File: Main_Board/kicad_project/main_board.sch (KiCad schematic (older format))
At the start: 0 parts

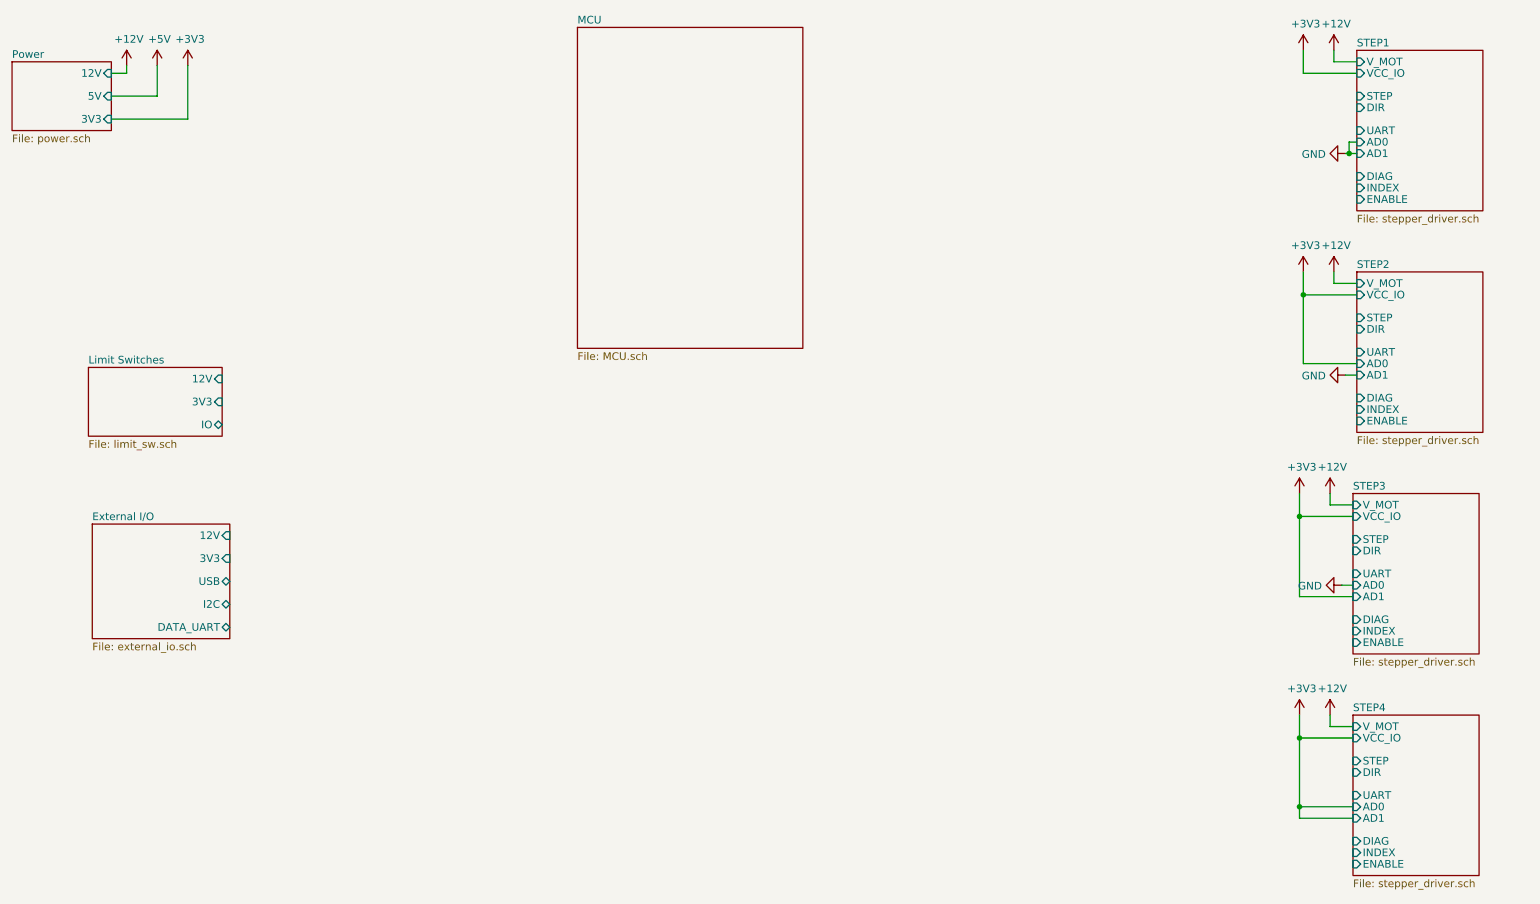
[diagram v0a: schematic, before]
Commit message: progress?
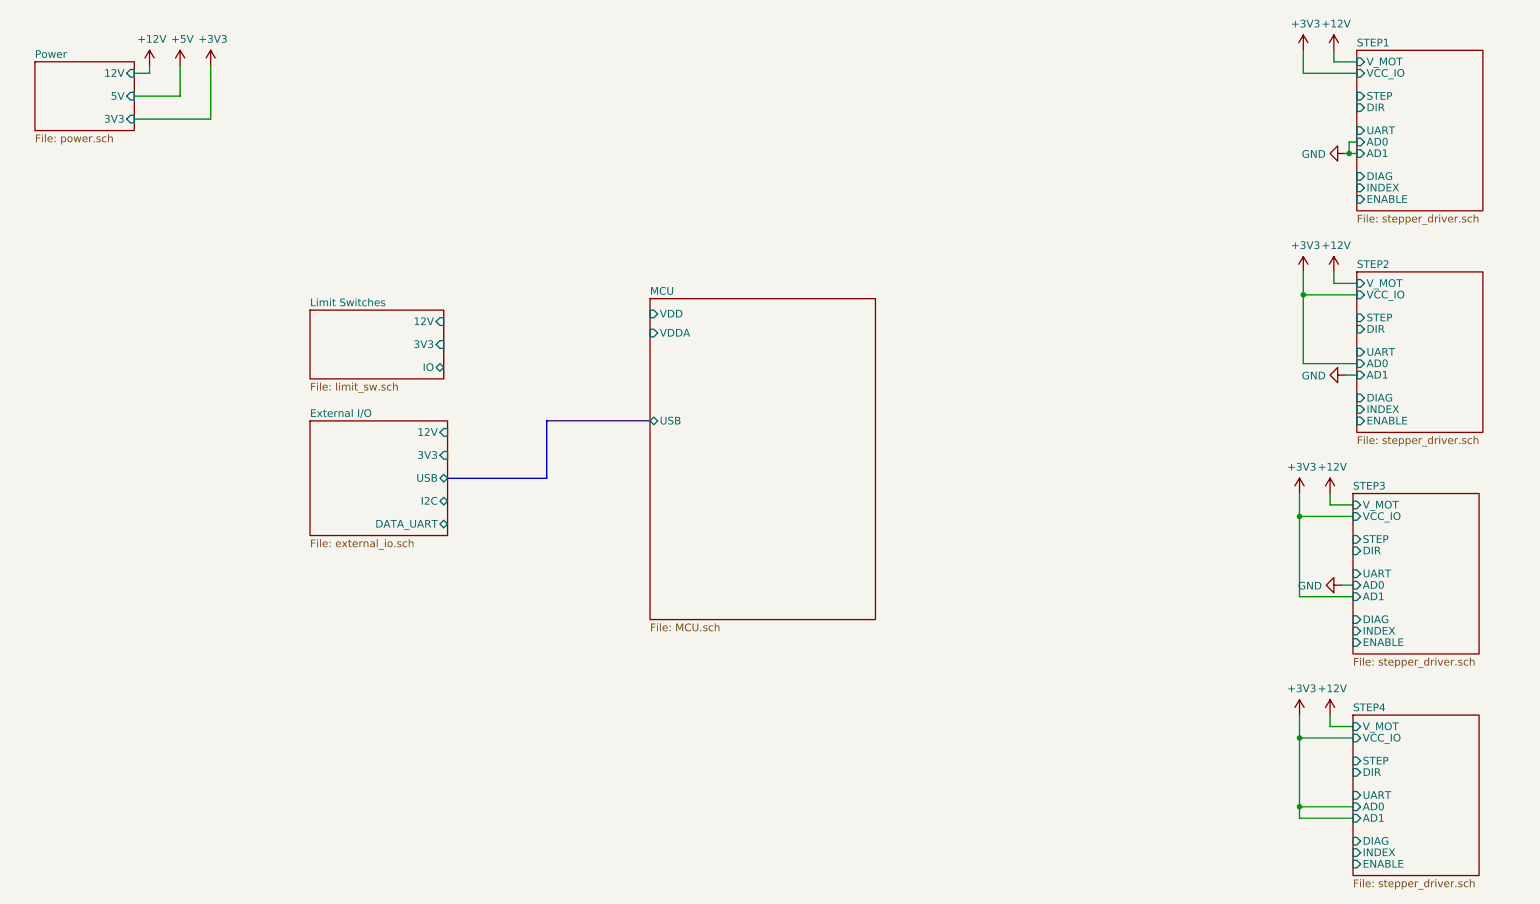
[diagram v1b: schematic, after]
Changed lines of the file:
@@
 	9500 1000 9500 850
 $Comp
-L power:+3V3 #PWR?
+L power:+3V3 #PWR06
 U 1 1 5F4AAFEB
 P 9500 850
-F 0 "#PWR?" H 9500 700 50  0001 C CNN
+F 0 "#PWR06" H 9500 700 50  0001 C CNN
 F 1 "+3V3" H 9515 1023 50  0000 C CNN
 F 2 "" H 9500 850 50  0001 C CNN
@@
 	9500 2450 9500 2300
 $Comp
-L power:+3V3 #PWR?
+L power:+3V3 #PWR07
 U 1 1 5F4AC7A4
 P 9500 2300
-F 0 "#PWR?" H 9500 2150 50  0001 C CNN
+F 0 "#PWR07" H 9500 2150 50  0001 C CNN
 F 1 "+3V3" H 9515 2473 50  0000 C CNN
 F 2 "" H 9500 2300 50  0001 C CNN
@@
 	9475 3900 9475 3750
 $Comp
-L power:+3V3 #PWR?
+L power:+3V3 #PWR04
 U 1 1 5F4AD226
 P 9475 3750
-F 0 "#PWR?" H 9475 3600 50  0001 C CNN
+F 0 "#PWR04" H 9475 3600 50  0001 C CNN
 F 1 "+3V3" H 9490 3923 50  0000 C CNN
 F 2 "" H 9475 3750 50  0001 C CNN
@@
 	9475 5350 9475 5200
 $Comp
-L power:+3V3 #PWR?
+L power:+3V3 #PWR05
 U 1 1 5F4ADFB4
 P 9475 5200
-F 0 "#PWR?" H 9475 5050 50  0001 C CNN
+F 0 "#PWR05" H 9475 5050 50  0001 C CNN
 F 1 "+3V3" H 9490 5373 50  0000 C CNN
 F 2 "" H 9475 5200 50  0001 C CNN
@@
 $EndComp
 $Sheet
-S 1050 925  650  450
+S 1200 925  650  450
 U 5F4D5F3E
 F0 "Power" 50
 F1 "power.sch" 50
-F2 "3V3" I R 1700 1300 50
-F3 "12V" I R 1700 1000 50
-F4 "5V" I R 1700 1150 50
-$EndSheet
-$Comp
-L power:+12V #PWR?
+F2 "3V3" I R 1850 1300 50
+F3 "12V" I R 1850 1000 50
+F4 "5V" I R 1850 1150 50
+$EndSheet
+$Comp
+L power:+12V #PWR09
 U 1 1 5F5780D9
 P 9675 5200
-F 0 "#PWR?" H 9675 5050 50  0001 C CNN
+F 0 "#PWR09" H 9675 5050 50  0001 C CNN
 F 1 "+12V" H 9690 5373 50  0000 C CNN
 F 2 "" H 9675 5200 50  0001 C CNN
@@
 $EndComp
 $Comp
-L power:+12V #PWR?
+L power:+12V #PWR08
 U 1 1 5F578445
 P 9675 3750
-F 0 "#PWR?" H 9675 3600 50  0001 C CNN
+F 0 "#PWR08" H 9675 3600 50  0001 C CNN
 F 1 "+12V" H 9690 3923 50  0000 C CNN
 F 2 "" H 9675 3750 50  0001 C CNN
@@
 $EndComp
 $Comp
-L power:+12V #PWR?
+L power:+12V #PWR011
 U 1 1 5F578DCD
 P 9700 2300
-F 0 "#PWR?" H 9700 2150 50  0001 C CNN
+F 0 "#PWR011" H 9700 2150 50  0001 C CNN
 F 1 "+12V" H 9715 2473 50  0000 C CNN
 F 2 "" H 9700 2300 50  0001 C CNN
@@
 $EndComp
 $Comp
-L power:+12V #PWR?
+L power:+12V #PWR010
 U 1 1 5F579C0A
 P 9700 850
-F 0 "#PWR?" H 9700 700 50  0001 C CNN
+F 0 "#PWR010" H 9700 700 50  0001 C CNN
 F 1 "+12V" H 9715 1023 50  0000 C CNN
 F 2 "" H 9700 850 50  0001 C CNN
@@
 $EndComp
 $Comp
-L power:+12V #PWR?
+L power:+12V #PWR01
 U 1 1 5F634CDC
-P 1800 950
-F 0 "#PWR?" H 1800 800 50  0001 C CNN
-F 1 "+12V" H 1815 1123 50  0000 C CNN
-F 2 "" H 1800 950 50  0001 C CNN
-F 3 "" H 1800 950 50  0001 C CNN
-	1    1800 950
-	1    0    0    -1
-$EndComp
-$Comp
-L power:+3V3 #PWR?
+P 1950 950
+F 0 "#PWR01" H 1950 800 50  0001 C CNN
+F 1 "+12V" H 1965 1123 50  0000 C CNN
+F 2 "" H 1950 950 50  0001 C CNN
+F 3 "" H 1950 950 50  0001 C CNN
+	1    1950 950
+	1    0    0    -1
+$EndComp
+$Comp
+L power:+3V3 #PWR03
 U 1 1 5F635D56
-P 2200 950
-F 0 "#PWR?" H 2200 800 50  0001 C CNN
-F 1 "+3V3" H 2215 1123 50  0000 C CNN
-F 2 "" H 2200 950 50  0001 C CNN
-F 3 "" H 2200 950 50  0001 C CNN
-	1    2200 950
-	1    0    0    -1
-$EndComp
-$Comp
-L power:+5V #PWR?
+P 2350 950
+F 0 "#PWR03" H 2350 800 50  0001 C CNN
+F 1 "+3V3" H 2365 1123 50  0000 C CNN
+F 2 "" H 2350 950 50  0001 C CNN
+F 3 "" H 2350 950 50  0001 C CNN
+	1    2350 950
+	1    0    0    -1
+$EndComp
+$Comp
+L power:+5V #PWR02
 U 1 1 5F636812
-P 2000 950
-F 0 "#PWR?" H 2000 800 50  0001 C CNN
-F 1 "+5V" H 2015 1123 50  0000 C CNN
-F 2 "" H 2000 950 50  0001 C CNN
-F 3 "" H 2000 950 50  0001 C CNN
-	1    2000 950
-	1    0    0    -1
-$EndComp
-Wire Wire Line
-	2200 950  2200 1300
-Wire Wire Line
-	2200 1300 1700 1300
-Wire Wire Line
-	1700 1150 2000 1150
-Wire Wire Line
-	2000 1150 2000 950
-Wire Wire Line
-	1700 1000 1800 1000
-Wire Wire Line
-	1800 1000 1800 950
+P 2150 950
+F 0 "#PWR02" H 2150 800 50  0001 C CNN
+F 1 "+5V" H 2165 1123 50  0000 C CNN
+F 2 "" H 2150 950 50  0001 C CNN
+F 3 "" H 2150 950 50  0001 C CNN
+	1    2150 950
+	1    0    0    -1
+$EndComp
+Wire Wire Line
+	2350 950  2350 1300
+Wire Wire Line
+	2350 1300 1850 1300
+Wire Wire Line
+	1850 1150 2150 1150
+Wire Wire Line
+	2150 1150 2150 950
+Wire Wire Line
+	1850 1000 1950 1000
+Wire Wire Line
+	1950 1000 1950 950
 Wire Wire Line
 	9825 4425 9475 4425
@@
 Connection ~ 9475 5800
 $Comp
-L power:GND #PWR?
+L power:GND #PWR013
 U 1 1 5F537589
 P 9775 1525
-F 0 "#PWR?" H 9775 1275 50  0001 C CNN
+F 0 "#PWR013" H 9775 1275 50  0001 C CNN
 F 1 "GND" V 9780 1397 50  0000 R CNN
 F 2 "" H 9775 1525 50  0001 C CNN
@@
 $EndComp
 $Comp
-L power:GND #PWR?
+L power:GND #PWR014
 U 1 1 5F53878C
 P 9775 2975
-F 0 "#PWR?" H 9775 2725 50  0001 C CNN
+F 0 "#PWR014" H 9775 2725 50  0001 C CNN
 F 1 "GND" V 9780 2847 50  0000 R CNN
 F 2 "" H 9775 2975 50  0001 C CNN
@@
 	9500 2900 9500 2450
 $Comp
-L power:GND #PWR?
+L power:GND #PWR012
 U 1 1 5F5393A9
 P 9750 4350
-F 0 "#PWR?" H 9750 4100 50  0001 C CNN
+F 0 "#PWR012" H 9750 4100 50  0001 C CNN
 F 1 "GND" V 9755 4222 50  0000 R CNN
 F 2 "" H 9750 4350 50  0001 C CNN
@@
 $EndComp
 $Sheet
-S 4750 700  1475 2100
+S 5225 2475 1475 2100
 U 5F5463C2
 F0 "MCU" 50
 F1 "MCU.sch" 50
-$EndSheet
-$Sheet
-S 1550 2925 875  450
+F2 "VDD" I L 5225 2575 50
+F3 "VDDA" I L 5225 2700 50
+F4 "USB" B L 5225 3275 50
+$EndSheet
+$Sheet
+S 3000 2550 875  450
 U 5F51A37F
 F0 "Limit Switches" 50
 F1 "limit_sw.sch" 50
-F2 "3V3" I R 2425 3150 50
-F3 "12V" I R 2425 3000 50
-F4 "IO" B R 2425 3300 50
-$EndSheet
-$Sheet
-S 1575 3950 900  750
+F2 "3V3" I R 3875 2775 50
+F3 "12V" I R 3875 2625 50
+F4 "IO" B R 3875 2925 50
+$EndSheet
+$Sheet
+S 3000 3275 900  750
 U 5F709561
 F0 "External I/O" 50
 F1 "external_io.sch" 50
-F2 "USB" B R 2475 4325 50
-F3 "3V3" I R 2475 4175 50
-F4 "12V" I R 2475 4025 50
-F5 "I2C" B R 2475 4475 50
-F6 "DATA_UART" B R 2475 4625 50
-$EndSheet
+F2 "USB" B R 3900 3650 50
+F3 "3V3" I R 3900 3500 50
+F4 "12V" I R 3900 3350 50
+F5 "I2C" B R 3900 3800 50
+F6 "DATA_UART" B R 3900 3950 50
+$EndSheet
+Wire Bus Line
+	3900 3650 4550 3650
+Wire Bus Line
+	4550 3650 4550 3275
+Wire Bus Line
+	4550 3275 5225 3275
 $EndSCHEMATC
